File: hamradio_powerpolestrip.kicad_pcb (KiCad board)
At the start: 2 copper layers, 145 x 50 mm, 27 parts, among them J1 Conn_01x02_Pin, J2 Conn_01x02_Pin, J3 Conn_01x02_Pin, J4 Conn_01x02_Pin, J5 Conn_01x02_Pin, J6 Conn_01x02_Pin, J7 Conn_01x02_Pin, J8 Conn_01x02_Pin

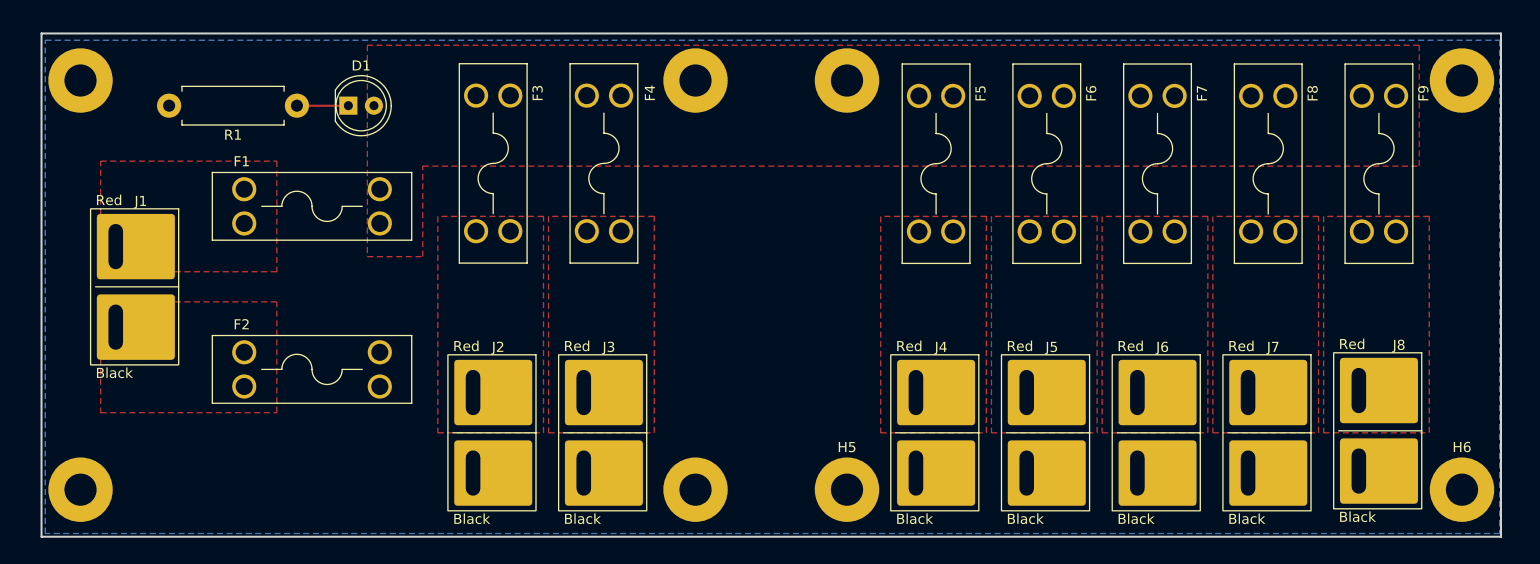
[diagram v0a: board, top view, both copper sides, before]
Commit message: updates
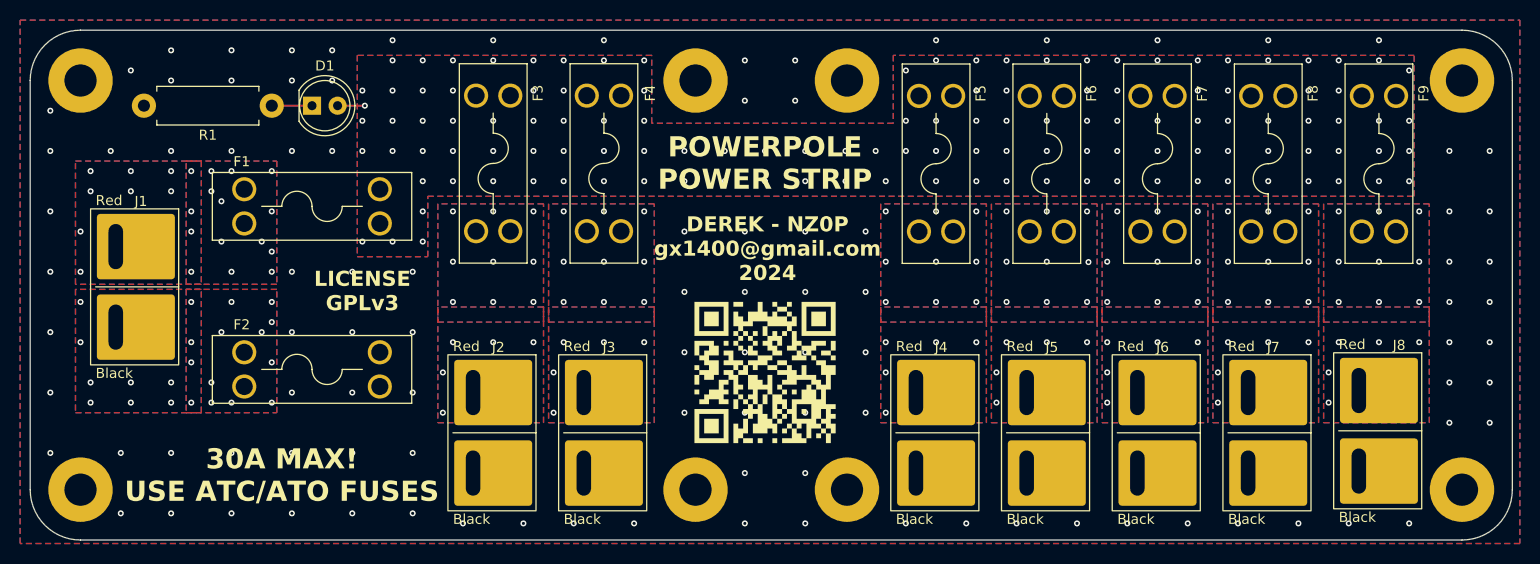
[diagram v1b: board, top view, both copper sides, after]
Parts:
- added G***: LOGO, Library:qrcode_15mm, F.Cu at (153.0, 109.0)
- moved D1 3.61 mm to (108.0, 82.5)
- moved R1 2.50 mm to (104.0, 82.5)
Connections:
- H1 pad 1: (no net) -> GND
- H2 pad 1: (no net) -> GND
- H3 pad 1: (no net) -> GND
- H4 pad 1: (no net) -> GND
- H5 pad 1: (no net) -> GND
- H6 pad 1: (no net) -> GND
- H7 pad 1: (no net) -> GND
- H8 pad 1: (no net) -> GND
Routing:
- net Net-(D1-K): track 0.00 -> 4.00 mm
- net +BATT: track 0.00 -> 2.71 mm, vias 0 -> 124
- net Net-(J8-Pin_1): vias 0 -> 14
- net Net-(J7-Pin_1): vias 0 -> 14
- net Net-(J6-Pin_1): vias 0 -> 14
- net Net-(J5-Pin_1): vias 0 -> 14
- net Net-(J4-Pin_1): vias 0 -> 14
- net Net-(J3-Pin_1): vias 0 -> 14
- net Net-(J2-Pin_1): vias 0 -> 14
- net Net-(J1-Pin_2): vias 0 -> 22
- net Net-(J1-Pin_1): vias 0 -> 23
- net GND: vias 0 -> 102
- added copper zone on B.Cu, net +BATT
- added copper zone on F.Cu, net GND
- added copper zone on B.Cu, net Net-(J1-Pin_1)
- added copper zone on B.Cu, net Net-(J1-Pin_2)
- added copper zone on B.Cu, net Net-(J2-Pin_1)
- added copper zone on B.Cu, net Net-(J3-Pin_1)
- added copper zone on B.Cu, net Net-(J4-Pin_1)
- added copper zone on B.Cu, net Net-(J5-Pin_1)
- added copper zone on B.Cu, net Net-(J6-Pin_1)
- added copper zone on B.Cu, net Net-(J7-Pin_1)
- added copper zone on B.Cu, net Net-(J8-Pin_1)
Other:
- board size 145 x 50 mm -> 147.2 x 50.7 mm
- board text added: "30A MAX! USE ATC/ATO FUSES"
- board text added: "DEREK - NZ0P gx1400@gmail.com 2024"
- board text added: "JLCJLCJLCJLC"
- board text added: "LICENSE GPLv3"
- board text added: "POWERPOLE POWER STRIP"
